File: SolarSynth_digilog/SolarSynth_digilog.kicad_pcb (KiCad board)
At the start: 2 copper layers, 60 x 89 mm, 30 parts, among them J1 OutputJack1, J2 Conn_01x01_Pin, J3 Conn_01x01_Pin, P1 PiezoDisc, P2 PiezoDisc, U1 74HC14, U2 MCP6002-xMC

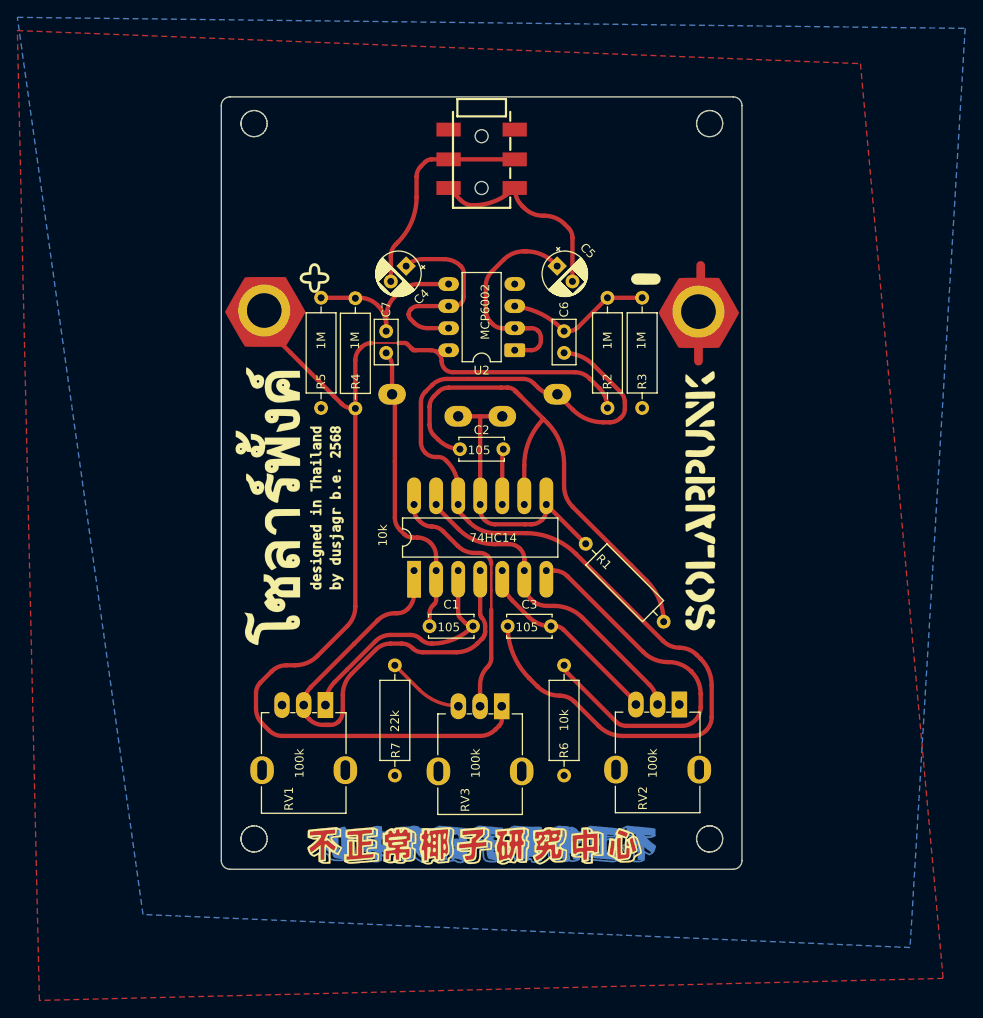
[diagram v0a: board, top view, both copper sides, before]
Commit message: added original digilog again and moved THT-Version to a new folder
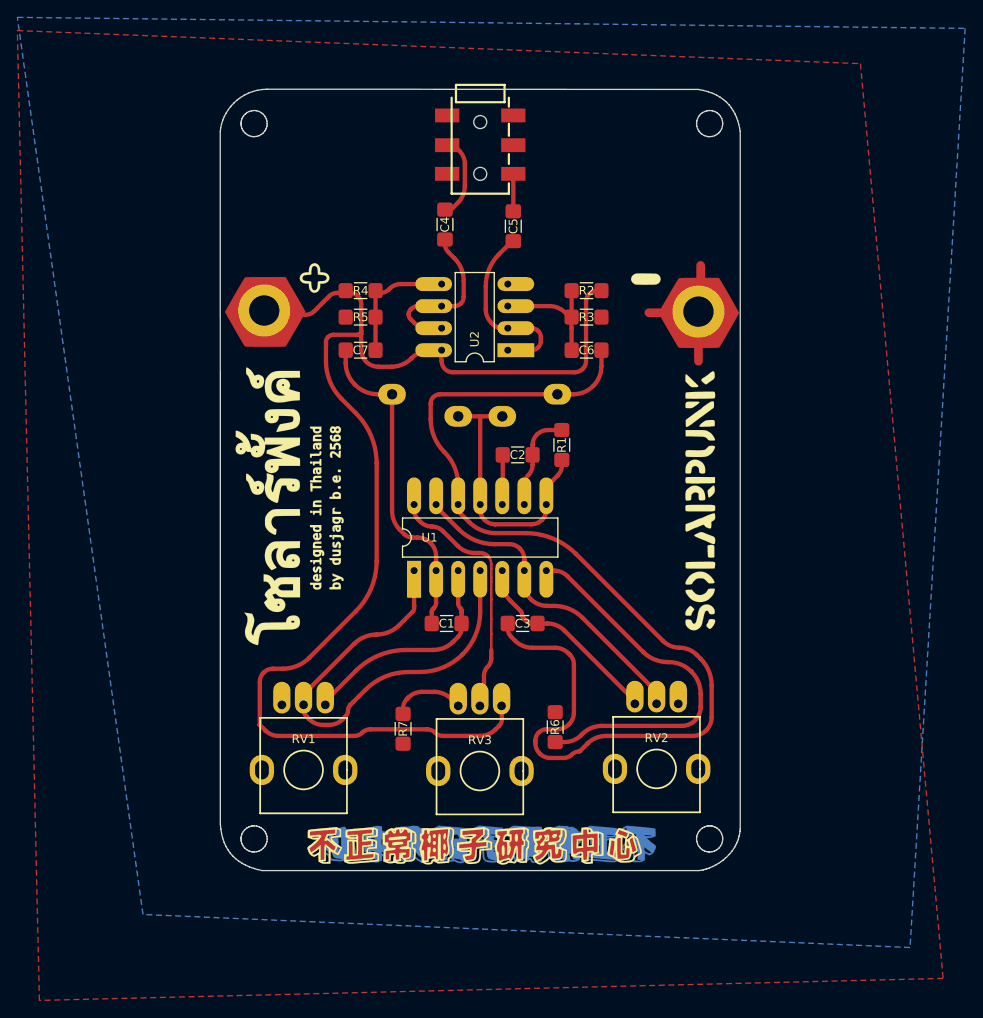
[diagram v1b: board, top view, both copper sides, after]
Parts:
- added edge1: 5VBoard, 007_dusjagr:board_digilog, F.Cu at (117.0, 74.4)
- C1, C2, C3: footprint Capacitor_THT:C_Disc_D5.0mm_W2.5mm_P5.00mm -> 007_dusjagr:C_1210_noGND
- C4, C5: footprint Capacitor_THT:CP_Radial_D5.0mm_P2.50mm -> 007_dusjagr:C_1210_noGND
- C6, C7: footprint Capacitor_THT:C_Disc_D5.0mm_W2.5mm_P2.50mm -> 007_dusjagr:C_1210_noGND
- J1: footprint 002_Solarpunk:AUDIO-JACK-3.5mm_SMD_noHole -> 007_dusjagr:AUDIO-JACK-3.5mm_SMD_Hole
- J2, J3: footprint 002_Solarpunk:SolarPad_VCC -> 007_dusjagr:SolarPad_VCC
- Pad1, Pad2, Pad3, Pad4: footprint 002_Solarpunk:SolderPad_small -> 007_dusjagr:SolderPad_small
- R1, R2, R3, R4, R5, R6, R7: footprint Resistor_THT:R_Axial_DIN0309_L9.0mm_D3.2mm_P12.70mm_Horizontal -> 007_dusjagr:R_1206_noGND
- RV1, RV2, RV3: footprint blinkyparts:Potentiometer_Alpha_RD901F-40-00D_Single_Vertical_bigger-holes -> 007_dusjagr:RD901F-ALPHA-3D_longpads
- U1: footprint 002_Solarpunk:DIP-14_W7.62mm_LongerPads -> 007_dusjagr:DIP-14_W7.62mm_LongerPads
- U2: footprint Package_DIP:DIP-8_W7.62mm_LongPads -> 007_dusjagr:DIP-8_W7.62mm_LongerPads
- moved R2 13.7 mm to (129.1, 52.8), turned to 180 degrees
- moved R4 13.6 mm to (103.1, 52.8), turned to 0 degrees
- moved R1 11.7 mm to (126.2, 70.6), turned to 90 degrees
- moved RV1 7.89 mm to (96.5, 108.1), turned to 180 degrees
- moved RV3 7.87 mm to (116.8, 108.2), turned to 180 degrees
- moved RV2 7.87 mm to (137.2, 107.9), turned to 180 degrees
- moved R7 7.38 mm to (108.0, 103.3)
- moved R6 7.20 mm to (125.5, 103.1), turned to 90 degrees
- moved C5 6.83 mm to (120.7, 45.4), turned to 90 degrees
- moved R3 6.79 mm to (129.1, 55.9), turned to 0 degrees
- moved C4 6.55 mm to (112.8, 45.2), turned to 90 degrees
- moved R5 5.07 mm to (103.1, 55.9), turned to 180 degrees
- moved C7 2.96 mm to (103.1, 59.7), turned to 0 degrees
- moved C6 2.61 mm to (129.1, 59.7), turned to 180 degrees
- moved C1 1.99 mm to (113.0, 91.2)
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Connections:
- J3 pad 1: GND -> (no net)
- RV1 pad 1: Net-(C1-Pad2) -> unconnected-(RV1-Pad1)
- RV1 pad 3: unconnected-(RV1-Pad3) -> Net-(C1-Pad2)
- RV2 pad 1: unconnected-(RV2-Pad1) -> Net-(C3-Pad2)
- RV2 pad 3: Net-(C3-Pad2) -> unconnected-(RV2-Pad3)
- RV3 pad 1: VCC -> Net-(R7-Pad1)
- RV3 pad 3: Net-(R7-Pad1) -> VCC
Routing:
- net Net-(C2-Pad2): track 64.8 -> 11.4 mm
- net Net-(C5-Pad2): track 23.9 -> 4.32 mm
- net VCC: track 125.0 -> 141.9 mm
- net Net-(C4-Pad2): track 26.0 -> 9.88 mm
- net Left: track 20.6 -> 14.4 mm
- net Net-(U2A--): track 29.5 -> 25.2 mm
- net Net-(RV1-Pad2): track 58.7 -> 55.0 mm
- net Right: track 17.8 -> 14.3 mm
- net Net-(Pad1-Pin_1): track 35.5 -> 38.9 mm
- net Net-(U2B--): track 22.3 -> 19.2 mm
- net Net-(Pad3-Pin_1): track 126.7 -> 123.8 mm
- net Net-(C1-Pad2): track 29.0 -> 26.2 mm
- net Net-(U1G-GND): track 45.4 -> 43.9 mm
- net Net-(Pad2-Pin_1): track 32.0 -> 30.9 mm
- net Net-(C3-Pad2): track 24.3 -> 23.5 mm
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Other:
- board size 60 x 89 mm -> 59.9 x 90 mm
- board text removed: "100k"
- board text removed: "105"
- board text removed: "10k"
- board text removed: "1M"
- board text removed: "22k"
- board text removed: "74HC14"
- board text removed: "MCP6002"
